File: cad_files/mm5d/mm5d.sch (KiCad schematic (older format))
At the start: 40 parts, among them P1 SCREW_CONN_1, P10 SCREW_CONN_1, P11 SCREW_CONN_1, P12 SCREW_CONN_1, P13 SCREW_CONN_1, P14 SCREW_CONN_1, P15 SCREW_CONN_1, P16 SCREW_CONN_1, P17 SCREW_CONN_1, P18 SCREW_CONN_1, P19 SCREW_CONN_1, P2 SCREW_CONN_1, P20 SCREW_CONN_1, P21 SCREW_CONN_1, P22 SCREW_CONN_1, P23 SCREW_CONN_1, P24 SCREW_CONN_1, P25 SCREW_CONN_1, P26 SCREW_CONN_1, P27 SCREW_CONN_1, P28 SCREW_CONN_1, P29 SCREW_CONN_1, P3 SCREW_CONN_1, P30 SCREW_CONN_1, P31 SCREW_CONN_1, P32 SCREW_CONN_1, P33 SCREW_CONN_1, P34 SCREW_CONN_1, P35 SCREW_CONN_1, P36 SCREW_CONN_1, P37 DB9, P4 SCREW_CONN_1, P5 SCREW_CONN_1, P6 SCREW_CONN_1, P7 SCREW_CONN_1, P8 SCREW_CONN_1, P9 SCREW_CONN_1, U4 Relay_panel, U5 Relay_panel

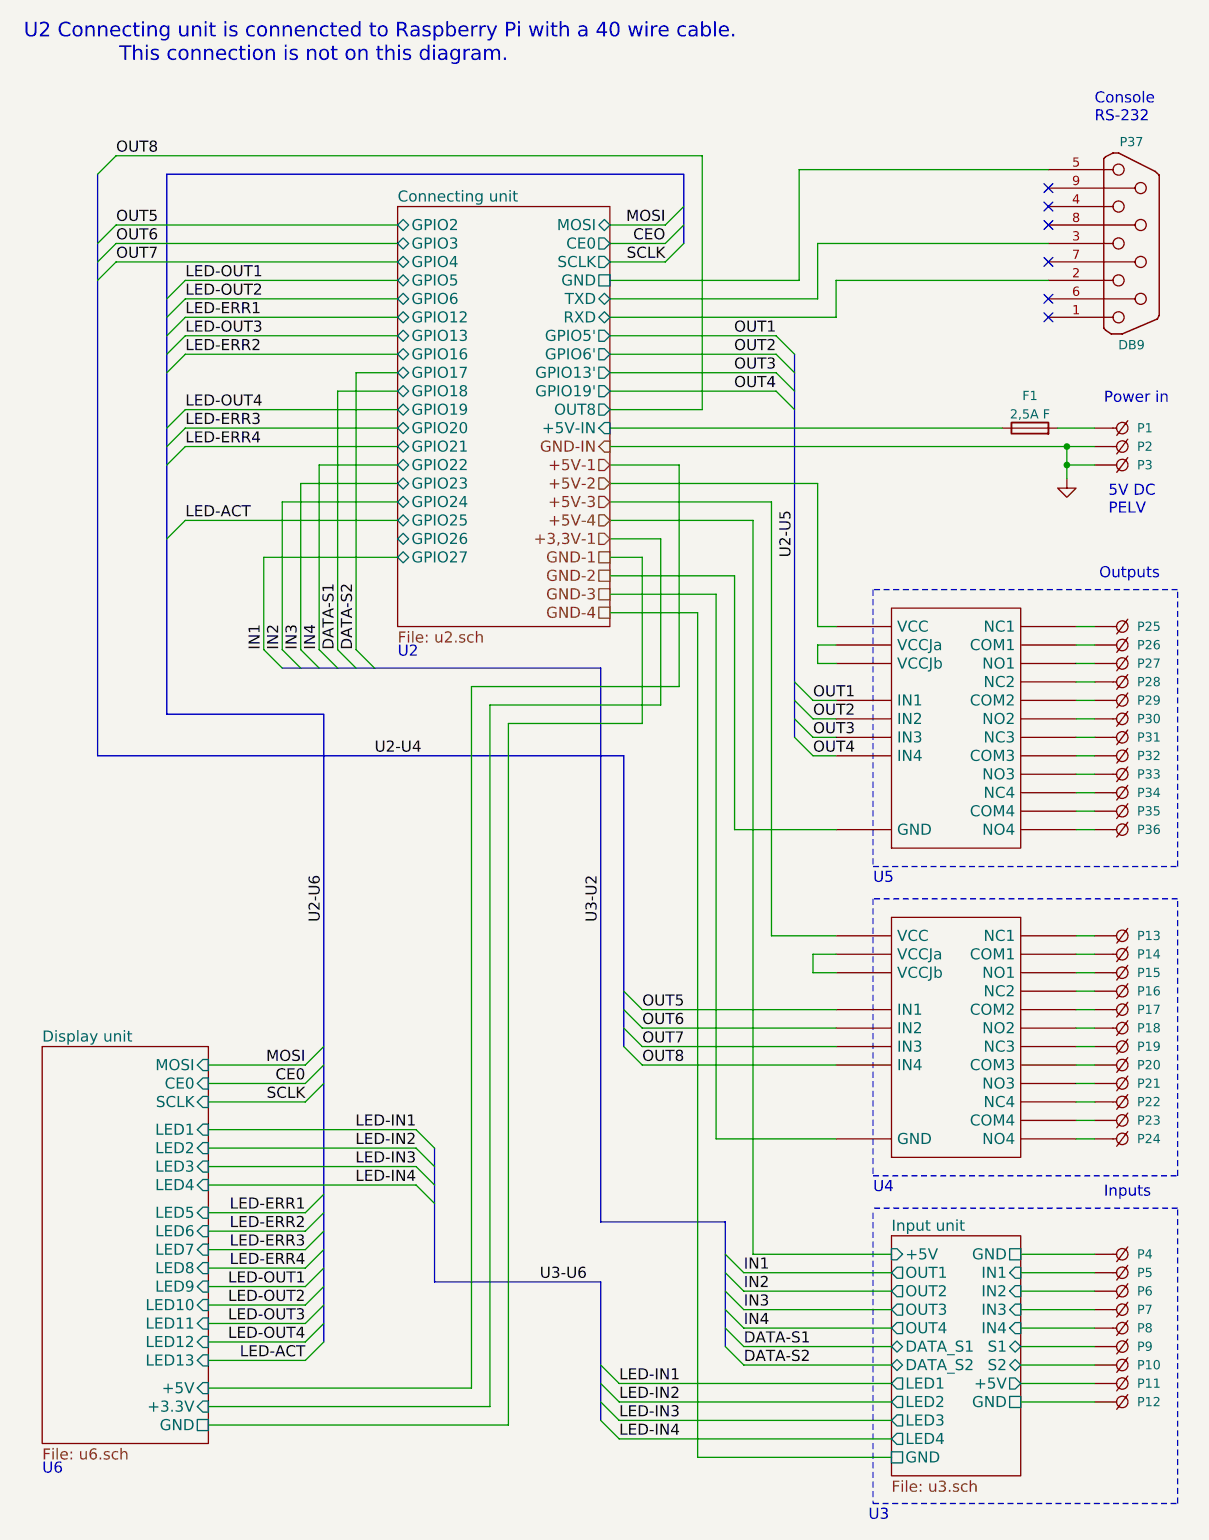
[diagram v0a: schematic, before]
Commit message: 190922
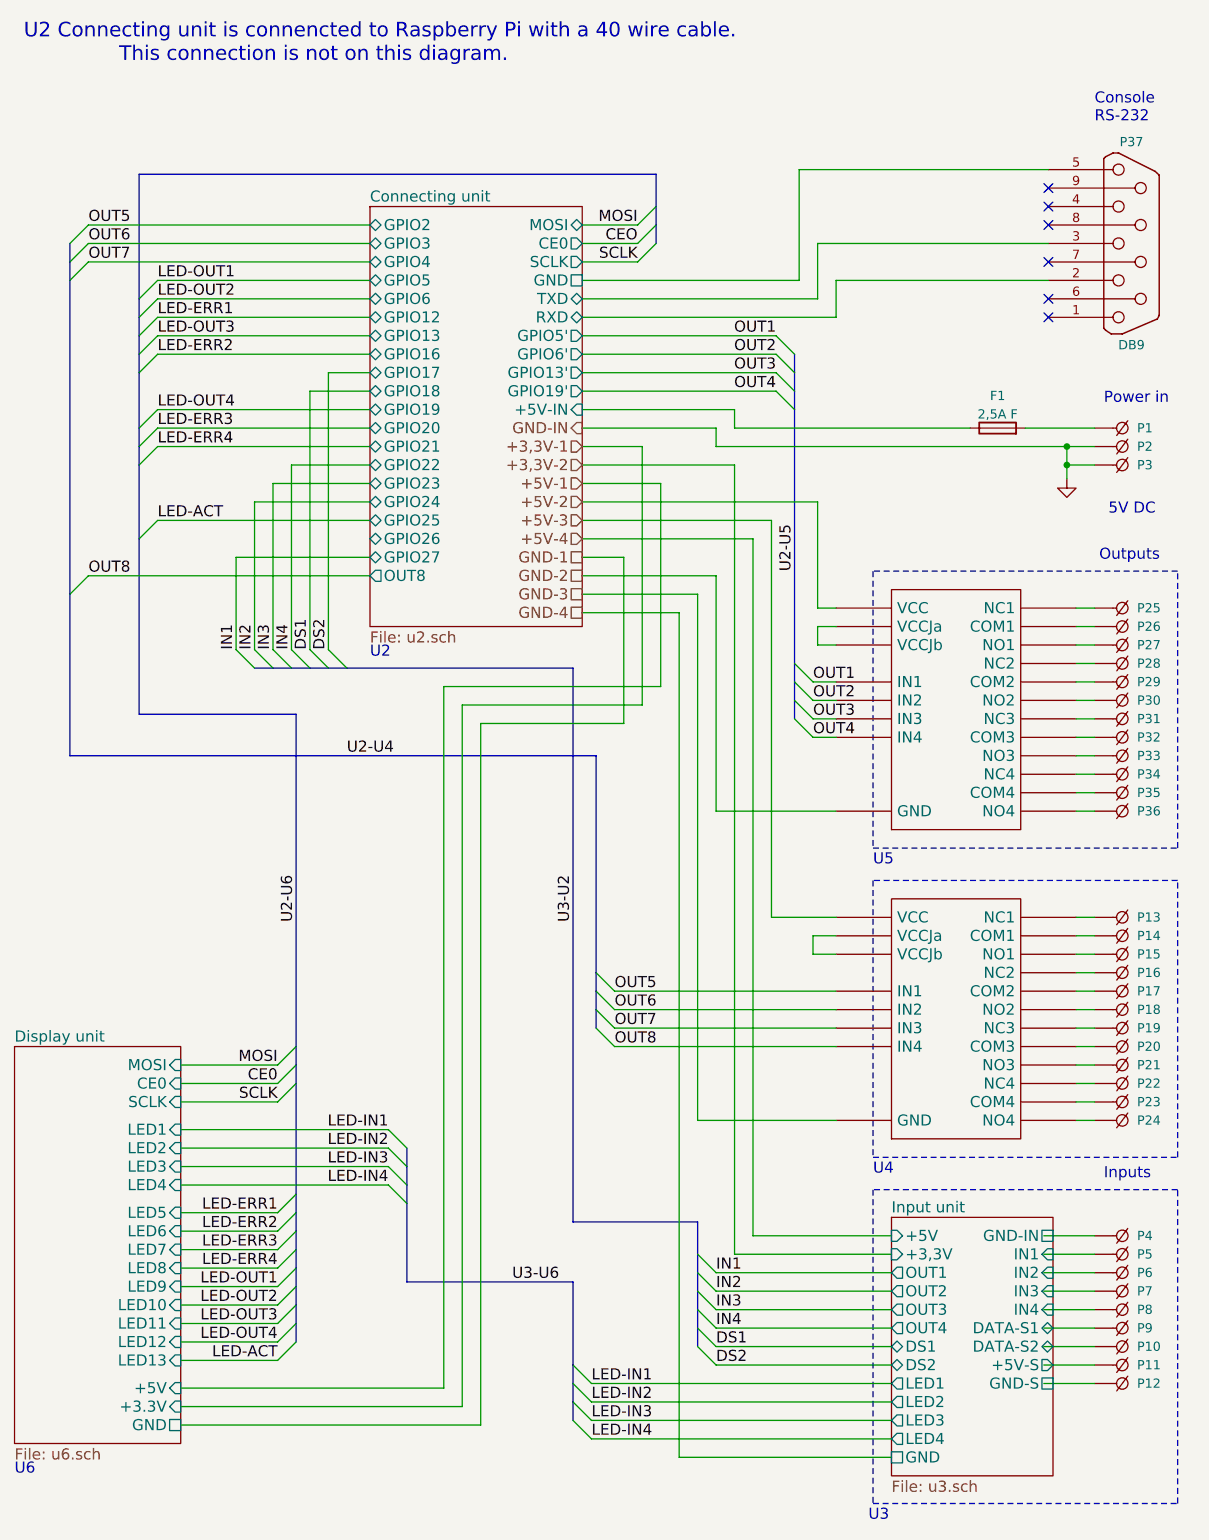
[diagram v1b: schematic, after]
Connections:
- net labels added: +3,3V-2, DS1, DS2
- net labels removed: DATA-S1, DATA-S2
- wire segments 154 -> 161
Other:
- note added: "5V DC"
- note removed: "5V DC\nPELV"
- moved on the sheet: F1, P10, P11, P12, P13, P14, P15, P16, P17, P18, P19, P20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
